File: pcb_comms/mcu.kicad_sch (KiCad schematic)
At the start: 28 parts, among them U2 STM32WLE5CCU6, Y3 32MHz

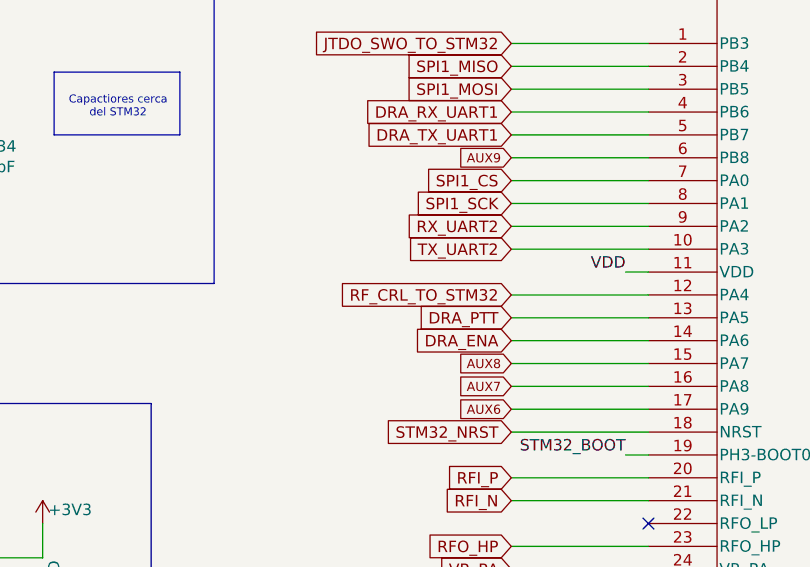
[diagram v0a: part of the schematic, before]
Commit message: Update pinout
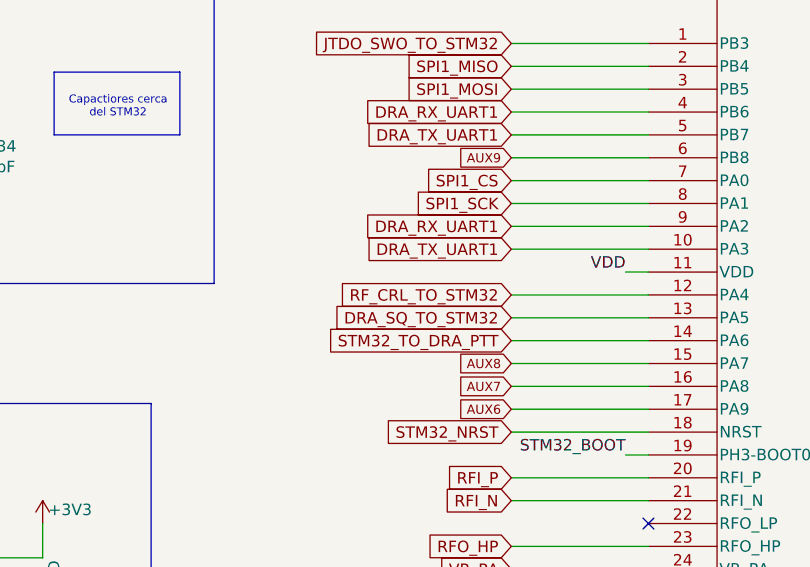
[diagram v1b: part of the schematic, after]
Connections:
- net RX_UART2 is gone; now on net DRA_RX_UART1: U2.9 (PA2)
- net TX_UART2 is gone; now on net DRA_TX_UART1: U2.10 (PA3)
- net DRA_ENA renamed STM32_TO_DRA_PTT
- net DRA_PTT renamed DRA_SQ_TO_STM32

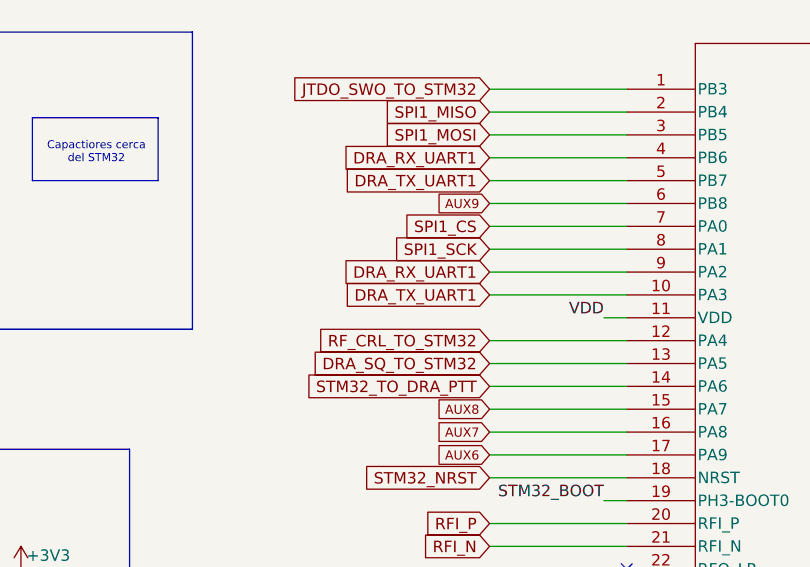
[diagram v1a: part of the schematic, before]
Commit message: Update pinout 2
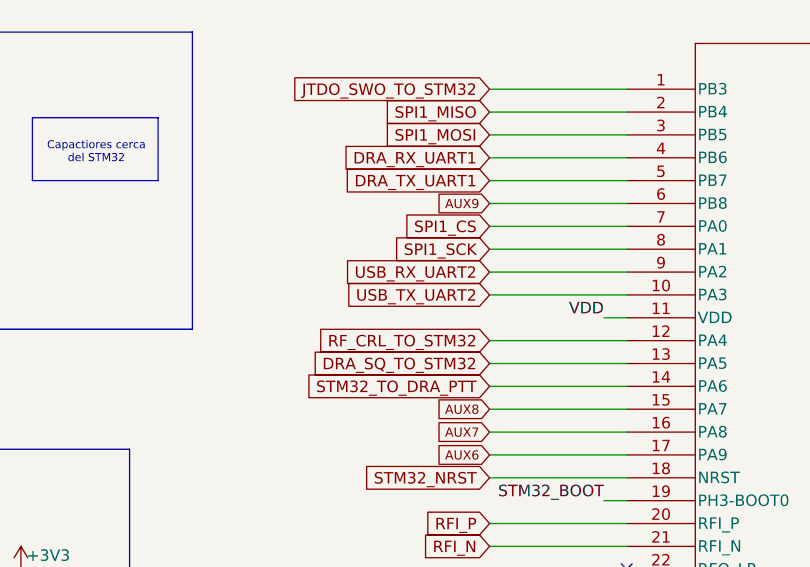
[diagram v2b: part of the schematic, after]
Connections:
- net DRA_RX_UART1: no longer U2.9 (PA2)
- net DRA_TX_UART1: no longer U2.10 (PA3)
- new net USB_RX_UART2: U2.9 (PA2)
- new net USB_TX_UART2: U2.10 (PA3)
